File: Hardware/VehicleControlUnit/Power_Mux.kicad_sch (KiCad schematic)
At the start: 6 parts, among them U2 TPS2117DRLR

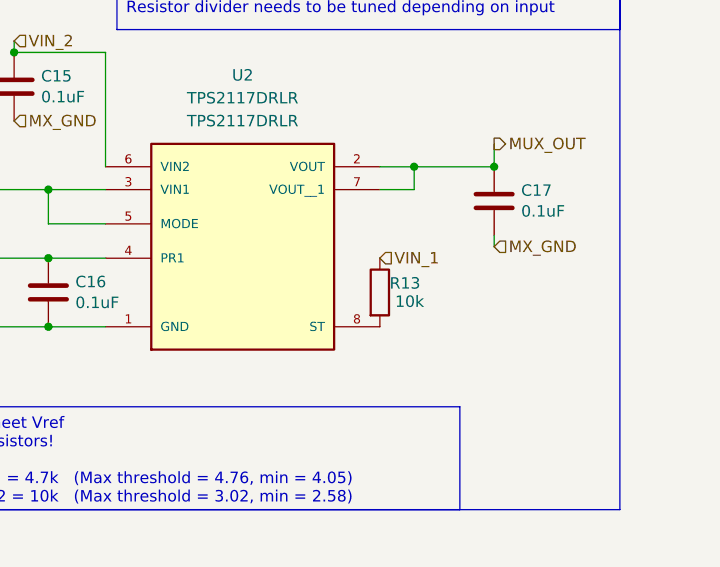
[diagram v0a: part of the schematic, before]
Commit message: i hate this moco, its so stupid why are we doign this.
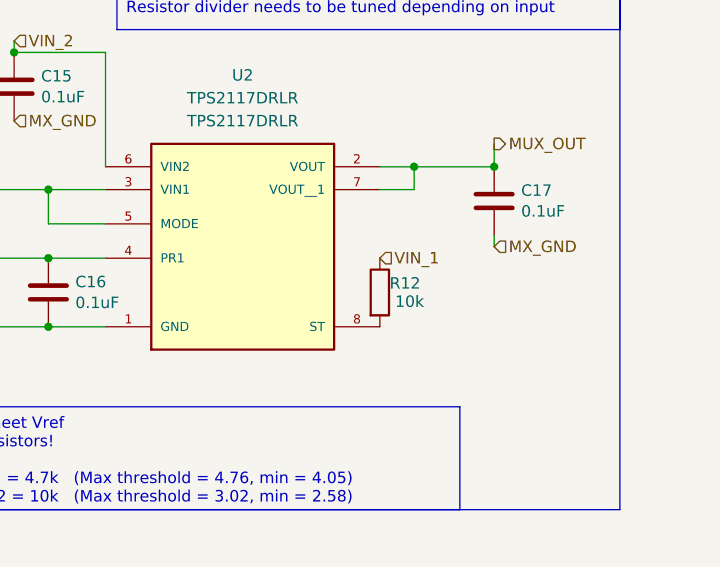
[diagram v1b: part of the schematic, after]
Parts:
- renumbered R13 to R12
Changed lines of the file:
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@@
 		(in_pos_files yes)
 		(dnp no)
-		(property "Reference" "R13"
+		(property "Reference" "R12"
 			(at 78.994 67.564 0)
 			(show_name no)
@@
 			(project "VehicleControlUnit"
 				(path "/e864fac9-3897-46c9-9101-6d5488c6cd3a/f16a8bc3-f058-4d27-badd-0afc148d009e/d4cd4986-72cf-4091-9d22-3ed3db5e35c5"
-					(reference "R13")
+					(reference "R12")
 					(unit 1)
 				)

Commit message: 70% tracing done
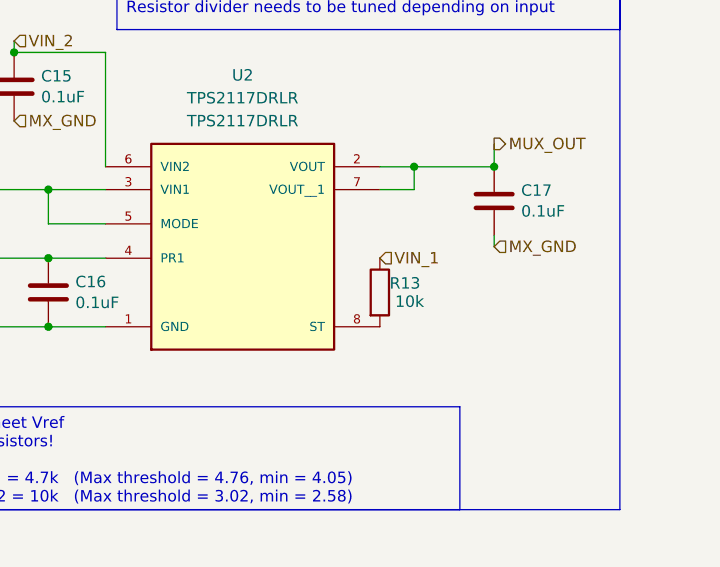
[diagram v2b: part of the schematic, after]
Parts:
- renumbered R12 to R13
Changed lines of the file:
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@@
 		(in_pos_files yes)
 		(dnp no)
-		(property "Reference" "R12"
+		(property "Reference" "R13"
 			(at 78.994 67.564 0)
 			(show_name no)
@@
 			(project "VehicleControlUnit"
 				(path "/e864fac9-3897-46c9-9101-6d5488c6cd3a/f16a8bc3-f058-4d27-badd-0afc148d009e/d4cd4986-72cf-4091-9d22-3ed3db5e35c5"
-					(reference "R12")
+					(reference "R13")
 					(unit 1)
 				)
